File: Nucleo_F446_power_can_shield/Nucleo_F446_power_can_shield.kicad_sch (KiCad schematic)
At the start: 8 parts

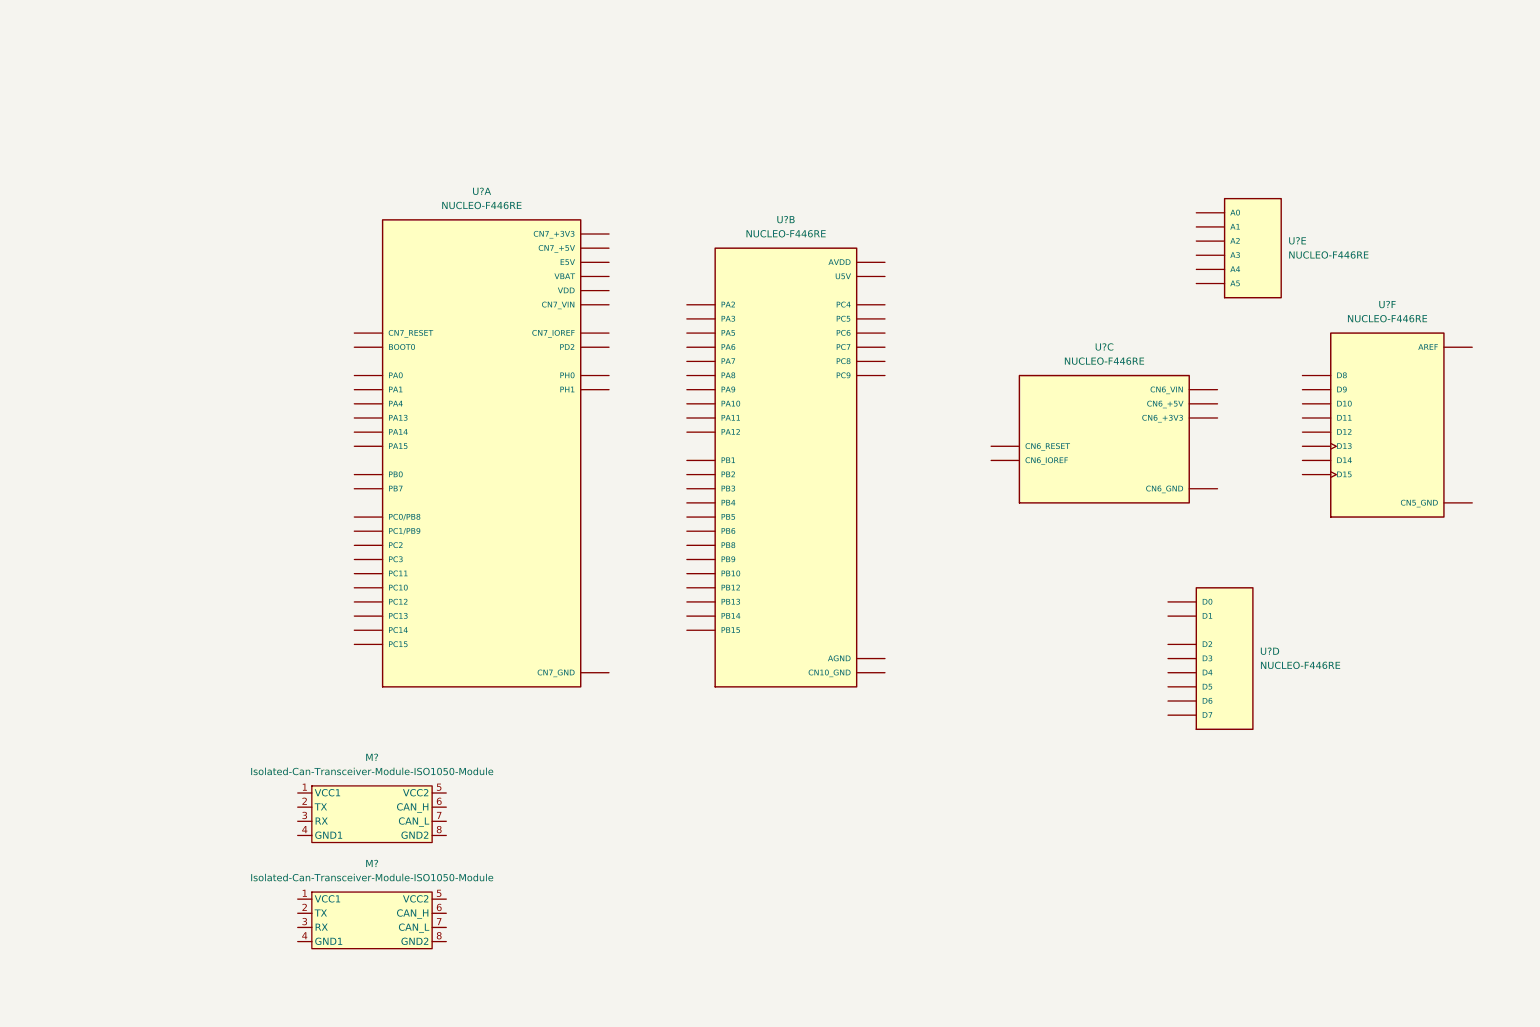
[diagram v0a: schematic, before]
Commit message: add lib
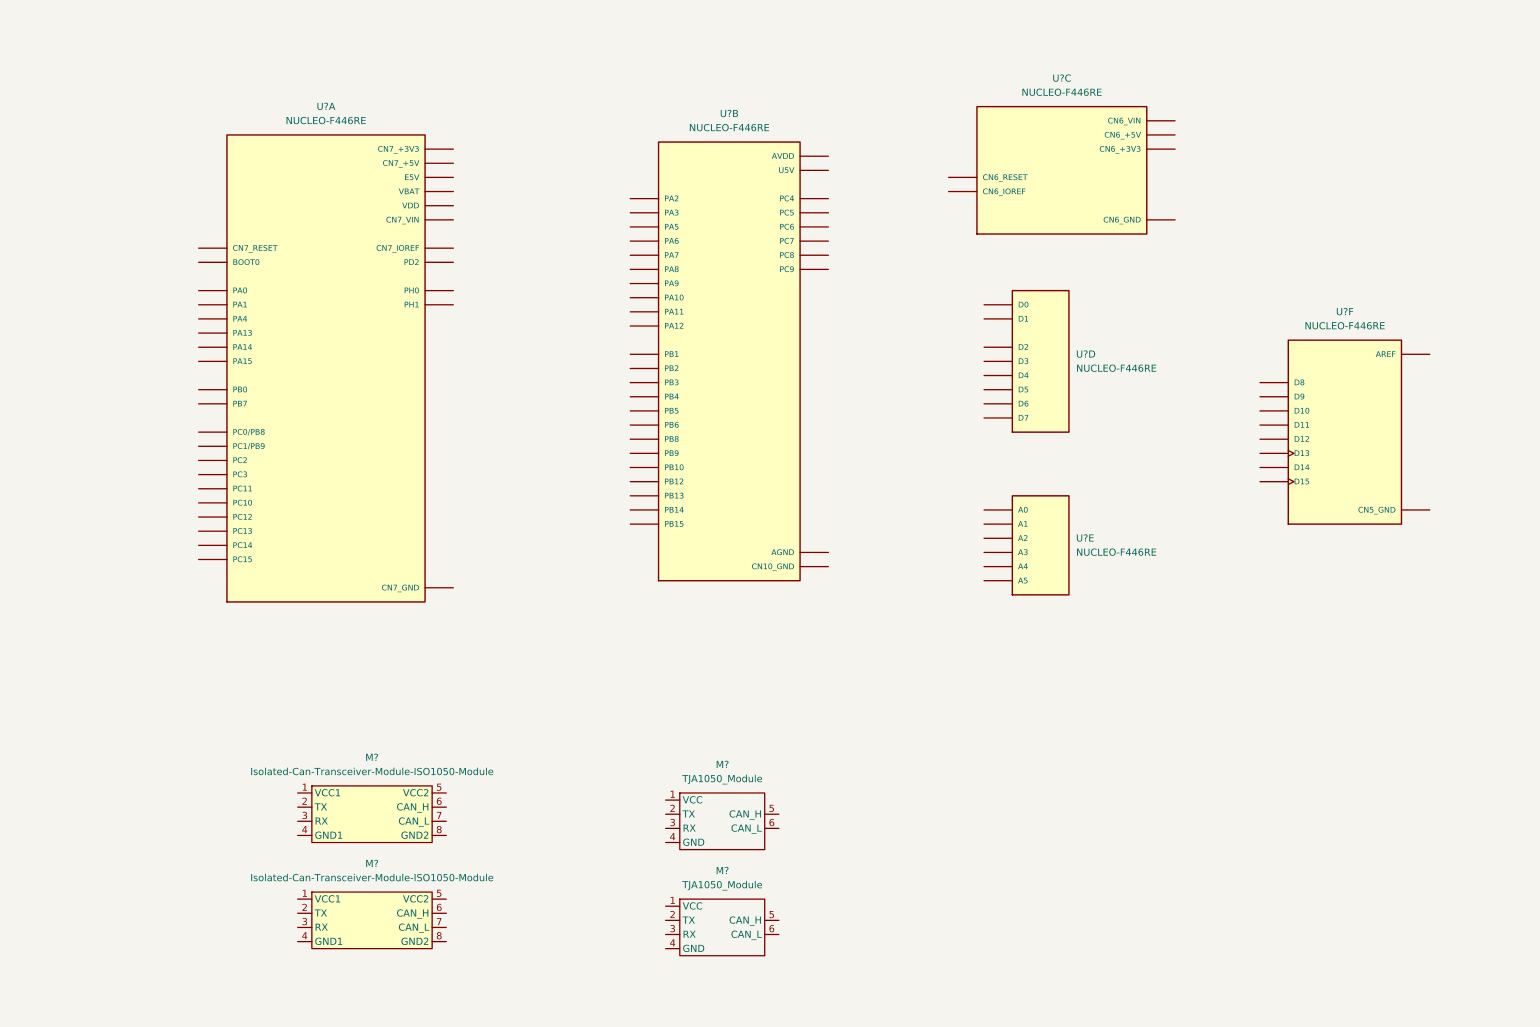
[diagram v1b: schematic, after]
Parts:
- added M? (x2): TJA1050_Module, PolyuRobotics:TJA1050_CAN_Module, symbol PolyuRobotics:TJA1050_Module
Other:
- moved on the sheet: U?A, U?B, U?C, U?D, U?E, U?F

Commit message: commit
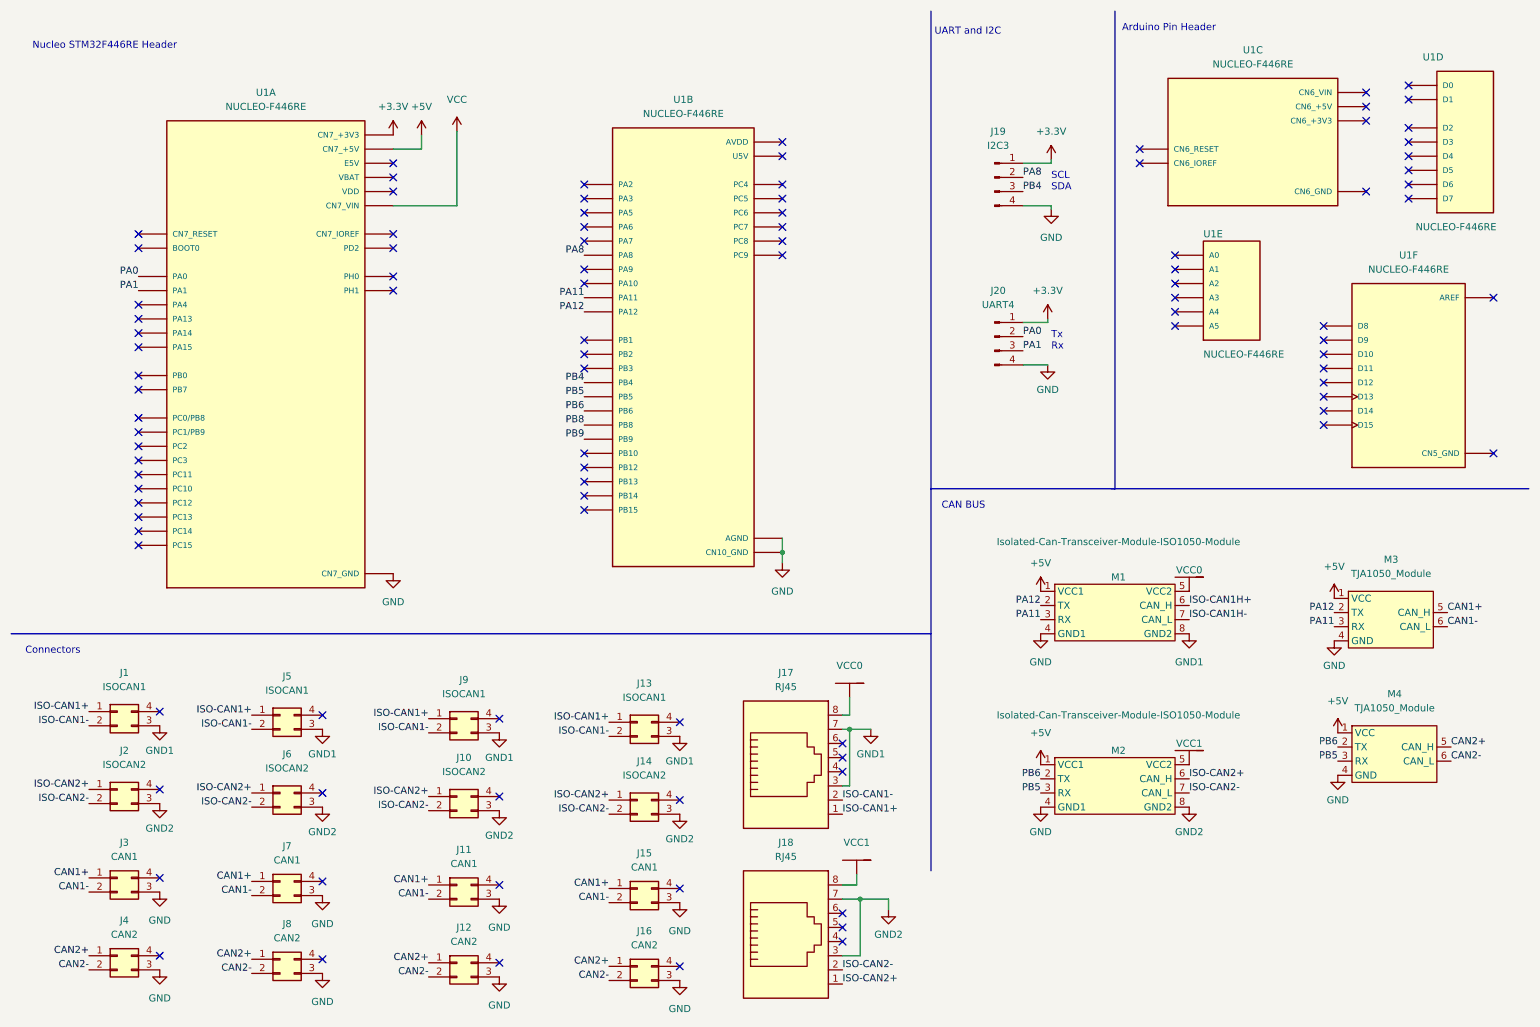
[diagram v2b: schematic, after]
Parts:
- removed M? (x2): Isolated-Can-Transceiver-Module-ISO1050-Module, symbol PolyuRobotics:Isolated-Can-Transceiver-Module-ISO1050-Module
- removed M? (x2): TJA1050_Module, PolyuRobotics:TJA1050_CAN_Module, symbol PolyuRobotics:TJA1050_Module
- added J1, J13, J5, J9: ISOCAN1, Connector_Molex:Molex_Micro-Fit_3.0_43045-0400_2x02_P3.00mm_Horizontal, symbol Connector_Generic:Conn_02x02_Counter_Clockwise
- added J10, J14, J2, J6: ISOCAN2, Connector_Molex:Molex_Micro-Fit_3.0_43045-0400_2x02_P3.00mm_Horizontal, symbol Connector_Generic:Conn_02x02_Counter_Clockwise
- added J11, J15, J3, J7: CAN1, Connector_Molex:Molex_Micro-Fit_3.0_43045-0400_2x02_P3.00mm_Horizontal, symbol Connector_Generic:Conn_02x02_Counter_Clockwise
- added J12, J16, J4, J8: CAN2, Connector_Molex:Molex_Micro-Fit_3.0_43045-0400_2x02_P3.00mm_Horizontal, symbol Connector_Generic:Conn_02x02_Counter_Clockwise
- added J17, J18: RJ45, Connector_RJ:RJ45_Amphenol_RJHSE5380, symbol Connector:RJ45
- added J19: I2C3, Connector_PinHeader_2.54mm:PinHeader_1x04_P2.54mm_Vertical, symbol Connector:Conn_01x04_Male
- added J20: UART4, Connector_PinHeader_2.54mm:PinHeader_1x04_P2.54mm_Vertical, symbol Connector:Conn_01x04_Male
- added M1, M2: Isolated-Can-Transceiver-Module-ISO1050-Module, PolyuRobotics:Isolated-Can-Transceiver-Module-ISO1050-Module, symbol PolyuRobotics:Isolated-Can-Transceiver-Module-ISO1050-Module
- added M3, M4: TJA1050_Module, PolyuRobotics:TJA1050_CAN_Module, symbol PolyuRobotics:TJA1050_Module
- U1: renamed from U?; footprint MODULE_NUCLEO-F446RE -> NUCLEO-F446RE:MODULE_NUCLEO-F446RE
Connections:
- net +3V3: now reaches U1.CN7_16 (CN7_+3V3)
- net +3V3: now also J19.1 (Pin_1), J20.1 (Pin_1)
- net +5V: now reaches U1.CN7_18 (CN7_+5V)
- net +5V: now also M1.1 (VCC1), M2.1 (VCC1), M3.1 (VCC), M4.1 (VCC)
- net GND: now reaches U1.CN7_19 (CN7_GND), U1.CN7_20 (CN7_GND), U1.CN7_22 (CN7_GND), U1.CN7_8 (CN7_GND)
- net GND: now also U1.CN10_20 (CN10_GND), U1.CN10_32 (AGND), U1.CN10_9 (CN10_GND), J11.3 (Pin_3), J12.3 (Pin_3), J15.3 (Pin_3), J16.3 (Pin_3), J19.4 (Pin_4), J20.4 (Pin_4), J3.3 (Pin_3), J4.3 (Pin_3), J7.3 (Pin_3), J8.3 (Pin_3), M1.4 (GND1), M2.4 (GND1), M3.4 (GND), M4.4 (GND)
- net VCC: now reaches U1.CN7_24 (CN7_VIN)
- net PA0: now reaches U1.CN7_28 (PA0)
- net PA0: now also J20.2 (Pin_2)
- net PA1: now reaches U1.CN7_30 (PA1)
- net PA1: now also J20.3 (Pin_3)
- net PA12: now reaches U1.CN10_12 (PA12)
- net PA12: now also M1.2 (TX), M3.2 (TX)
- net PA11: now reaches U1.CN10_14 (PA11)
- net PA11: now also M1.3 (RX), M3.3 (RX)
- net PB6: now reaches U1.CN10_17 (PB6)
- net PB6: now also M2.2 (TX), M4.2 (TX)
- net PA8: now reaches U1.CN10_23 (PA8)
- net PA8: now also J19.2 (Pin_2)
- net PB4: now reaches U1.CN10_27 (PB4)
- net PB4: now also J19.3 (Pin_3)
- net PB5: now reaches U1.CN10_29 (PB5)
- net PB5: now also M2.3 (RX), M4.3 (RX)
- net PB8: now reaches U1.CN10_3 (PB8)
- net PB9: now reaches U1.CN10_5 (PB9)
- new net CAN1+: J11.1 (Pin_1), J15.1 (Pin_1), J3.1 (Pin_1), J7.1 (Pin_1), M3.5 (CAN_H)
- new net CAN1-: J11.2 (Pin_2), J15.2 (Pin_2), J3.2 (Pin_2), J7.2 (Pin_2), M3.6 (CAN_L)
- new net CAN2+: J12.1 (Pin_1), J16.1 (Pin_1), J4.1 (Pin_1), J8.1 (Pin_1), M4.5 (CAN_H)
- new net CAN2-: J12.2 (Pin_2), J16.2 (Pin_2), J4.2 (Pin_2), J8.2 (Pin_2), M4.6 (CAN_L)
- new net GND1: J1.3 (Pin_3), J13.3 (Pin_3), J17.3, J17.7, J5.3 (Pin_3), J9.3 (Pin_3), M1.8 (GND2)
- new net GND2: J10.3 (Pin_3), J14.3 (Pin_3), J18.3, J18.7, J2.3 (Pin_3), J6.3 (Pin_3), M2.8 (GND2)
- new net ISO-CAN1+: J1.1 (Pin_1), J13.1 (Pin_1), J17.1, J5.1 (Pin_1), J9.1 (Pin_1)
- new net ISO-CAN1-: J1.2 (Pin_2), J13.2 (Pin_2), J17.2, J5.2 (Pin_2), J9.2 (Pin_2)
- new net ISO-CAN1H+: M1.6 (CAN_H)
- new net ISO-CAN1H-: M1.7 (CAN_L)
- new net ISO-CAN2+: J10.1 (Pin_1), J14.1 (Pin_1), J18.1, J2.1 (Pin_1), J6.1 (Pin_1), M2.6 (CAN_H)
- new net ISO-CAN2-: J10.2 (Pin_2), J14.2 (Pin_2), J18.2, J2.2 (Pin_2), J6.2 (Pin_2), M2.7 (CAN_L)
- new net VCC0: J17.8, M1.5 (VCC2)
- new net VCC1: J18.8, M2.5 (VCC2)
- no-connect marks 0 -> 100
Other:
- note added: "Arduino Pin Header"
- note added: "CAN BUS"
- note added: "Connectors"
- note added: "Nucleo STM32F446RE Header"
- note added: "SCL SDA"
- note added: "Tx Rx"
- note added: "UART and I2C"
- moved on the sheet: U1A, U1B, U1C, U1D, U1E, U1F
